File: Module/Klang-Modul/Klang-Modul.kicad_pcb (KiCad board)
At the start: 2 copper layers, 120.5 x 65 mm, 46 parts, among them J1 Conn_01x07, T808 BC547, T814 BC547, T828 BC547, T834 BC547

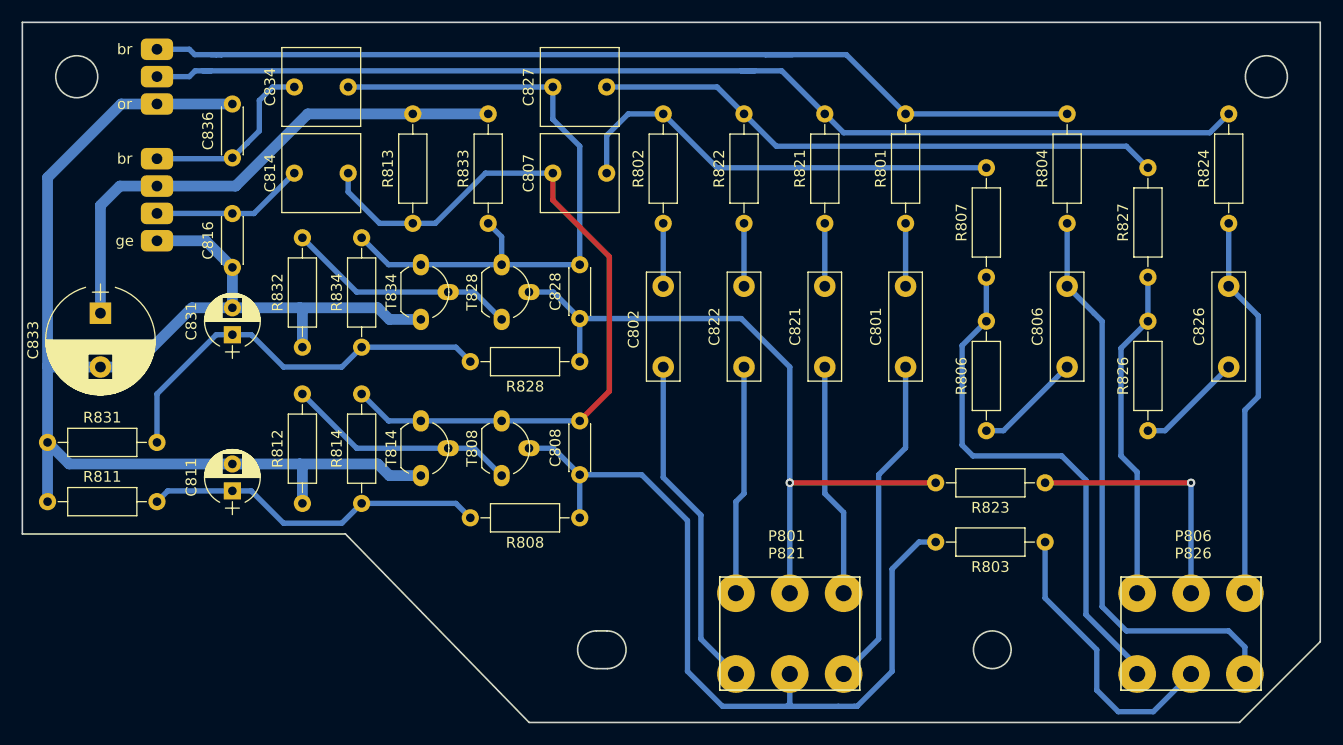
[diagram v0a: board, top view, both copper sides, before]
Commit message: A bunch of new modules added.
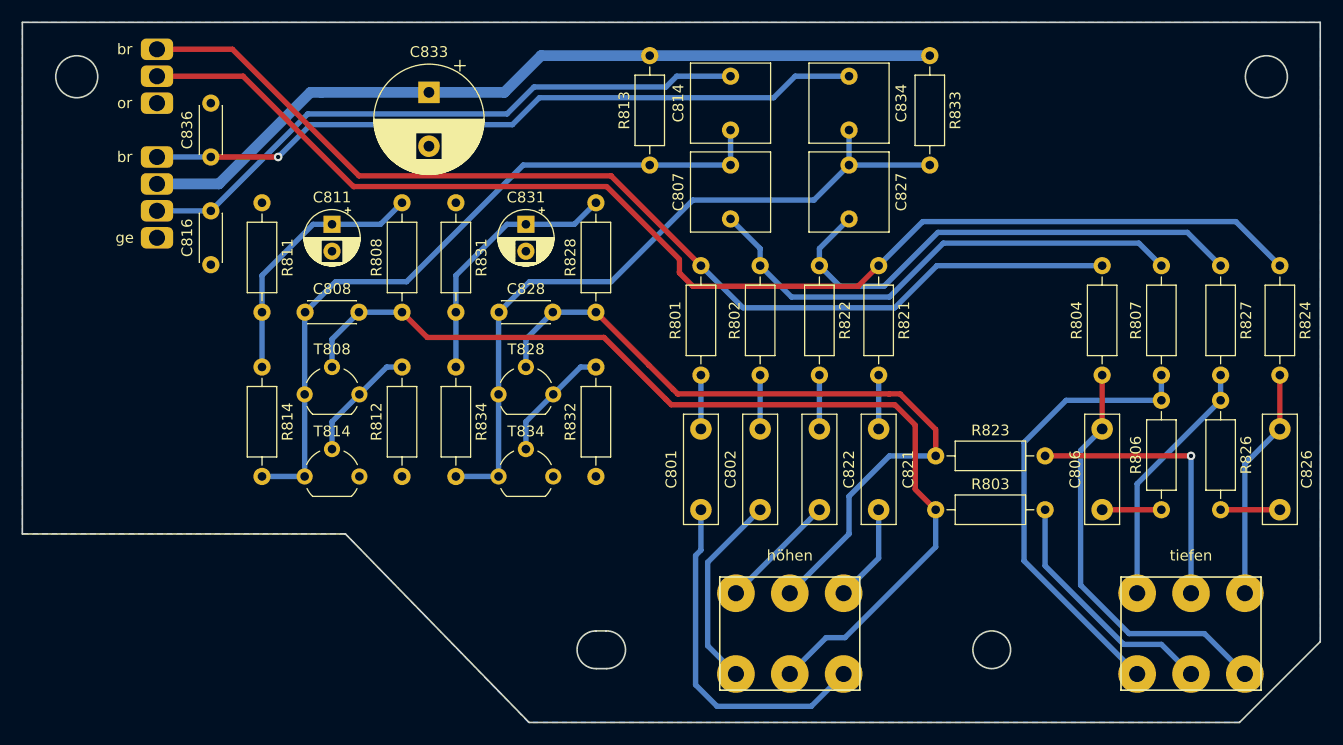
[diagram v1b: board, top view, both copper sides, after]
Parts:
- C801, C802, C806, C821, C822, C826: footprint Capacitors_THT:C_Rect_L10.0mm_W3.0mm_P7.50mm_MKS4 -> Capacitor_THT:C_Rect_L10.0mm_W3.0mm_P7.50mm_MKS4
- C807, C814, C827, C834: footprint Capacitors_THT:C_Rect_L7.2mm_W7.2mm_P5.00mm_FKS2_FKP2_MKS2_MKP2 -> Capacitor_THT:C_Rect_L7.2mm_W7.2mm_P5.00mm_FKS2_FKP2_MKS2_MKP2
- C808, C816, C828: footprint Capacitors_THT:C_Disc_D4.3mm_W1.9mm_P5.00mm -> Capacitor_THT:C_Disc_D4.3mm_W1.9mm_P5.00mm
- C811, C831: footprint Capacitors_THT:CP_Radial_D5.0mm_P2.50mm -> Capacitor_THT:CP_Radial_D5.0mm_P2.50mm
- C833: footprint Capacitors_THT:CP_Radial_D10.0mm_P5.00mm -> Capacitor_THT:CP_Radial_D10.0mm_P5.00mm
- C836: value 22nF -> 2.2nF; footprint Capacitors_THT:C_Disc_D4.3mm_W1.9mm_P5.00mm -> Capacitor_THT:C_Disc_D4.3mm_W1.9mm_P5.00mm
- R801, R802, R803, R804, R806, R807, R808, R811, R812, R813, R814, R821, R822, R823, R824, R826, R827, R828, R831, R832, R833, R834: footprint Resistors_THT:R_Axial_DIN0207_L6.3mm_D2.5mm_P10.16mm_Horizontal -> Resistor_THT:R_Axial_DIN0207_L6.3mm_D2.5mm_P10.16mm_Horizontal
- T808, T814, T828, T834: footprint TO_SOT_Packages_THT:TO-92_Molded_Wide_Oval -> Package_TO_SOT_THT:TO-92_Wide
- moved C834 46.7 mm to (116.2, 40.0), turned to 90 degrees
- moved R833 41.4 mm to (123.8, 33.1)
- moved C833 36.7 mm to (77.2, 36.5)
- moved C814 35.7 mm to (105.2, 40.0), turned to 90 degrees
- moved R831 30.3 mm to (79.8, 56.9), turned to 90 degrees
- moved R832 29.8 mm to (92.8, 62.0)
- moved C831 29.1 mm to (86.2, 48.8), turned to -90 degrees
- moved C827 28.4 mm to (116.2, 43.2), turned to -90 degrees
- moved C808 27.4 mm to (65.8, 56.9), turned to 0 degrees
- moved C811 26.4 mm to (68.2, 48.8), turned to -90 degrees
- moved R808 25.2 mm to (74.8, 56.9), turned to 90 degrees
- moved R834 23.8 mm to (79.8, 72.2), turned to 90 degrees
- moved R801 23.7 mm to (102.5, 62.8)
- moved C801 23.2 mm to (102.5, 75.2)
- moved R813 22.7 mm to (97.8, 33.1)
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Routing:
- net GND: track 142.9 -> 0.00 mm
- net OUT_R: track 17.2 -> 67.4 mm, vias 0 -> 1
- net OUT_L: track 14.3 -> 58.4 mm
- net +24V: track 49.5 -> 76.7 mm
- net Net-(T808-B): track 74.9 -> 92.6 mm
- net Net-(C806-Pad2): track 54.2 -> 39.0 mm
- net Net-(C826-Pad2): track 36.0 -> 21.6 mm
- net Net-(C831-Pad1): track 38.4 -> 24.3 mm
- net Net-(C802-Pad2): track 31.3 -> 18.4 mm
- net Net-(C821-Pad1): track 21.7 -> 9.10 mm
- net IN_R: track 104.8 -> 117.2 mm
- net Net-(T828-E): track 21.6 -> 11.1 mm
- net Net-(T808-E): track 21.6 -> 11.1 mm
- net Net-(C822-Pad2): track 21.3 -> 11.0 mm
- net IN_L: track 90.5 -> 99.3 mm
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- added copper zone on B.Cu, net GND
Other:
- outline, holes or cut-outs redrawn
- net class Default removed
- board text added: "+24V"
- board text added: "GND"
- board text added: "L"
- board text added: "R"
- board text added: "höhen"
- board text added: "tiefen"
- board text removed: "P801 P821"
- board text removed: "P806 P826"
